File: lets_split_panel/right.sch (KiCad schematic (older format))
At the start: 52 parts, among them J5 Speaker, J6 ISP, J8 WS2812>, P5 USB_OTG, P6 >WS2812, P8 Conn_01x04, SW25 Socket, SW26 Socket, SW27 Socket, SW28 Socket, SW29 Socket, SW30 Socket, SW31 Socket, SW32 Socket, SW33 Socket, SW34 Socket, SW35 Socket, SW36 Socket, SW37 Socket, SW38 Socket, SW39 Socket, SW40 Socket, SW41 Socket, SW42 Socket, SW43 Socket, SW44 Socket, SW45 Socket, SW46 Socket, SW47 Socket, SW48 Socket, U2 ATMega32U4, Y2 Crystal

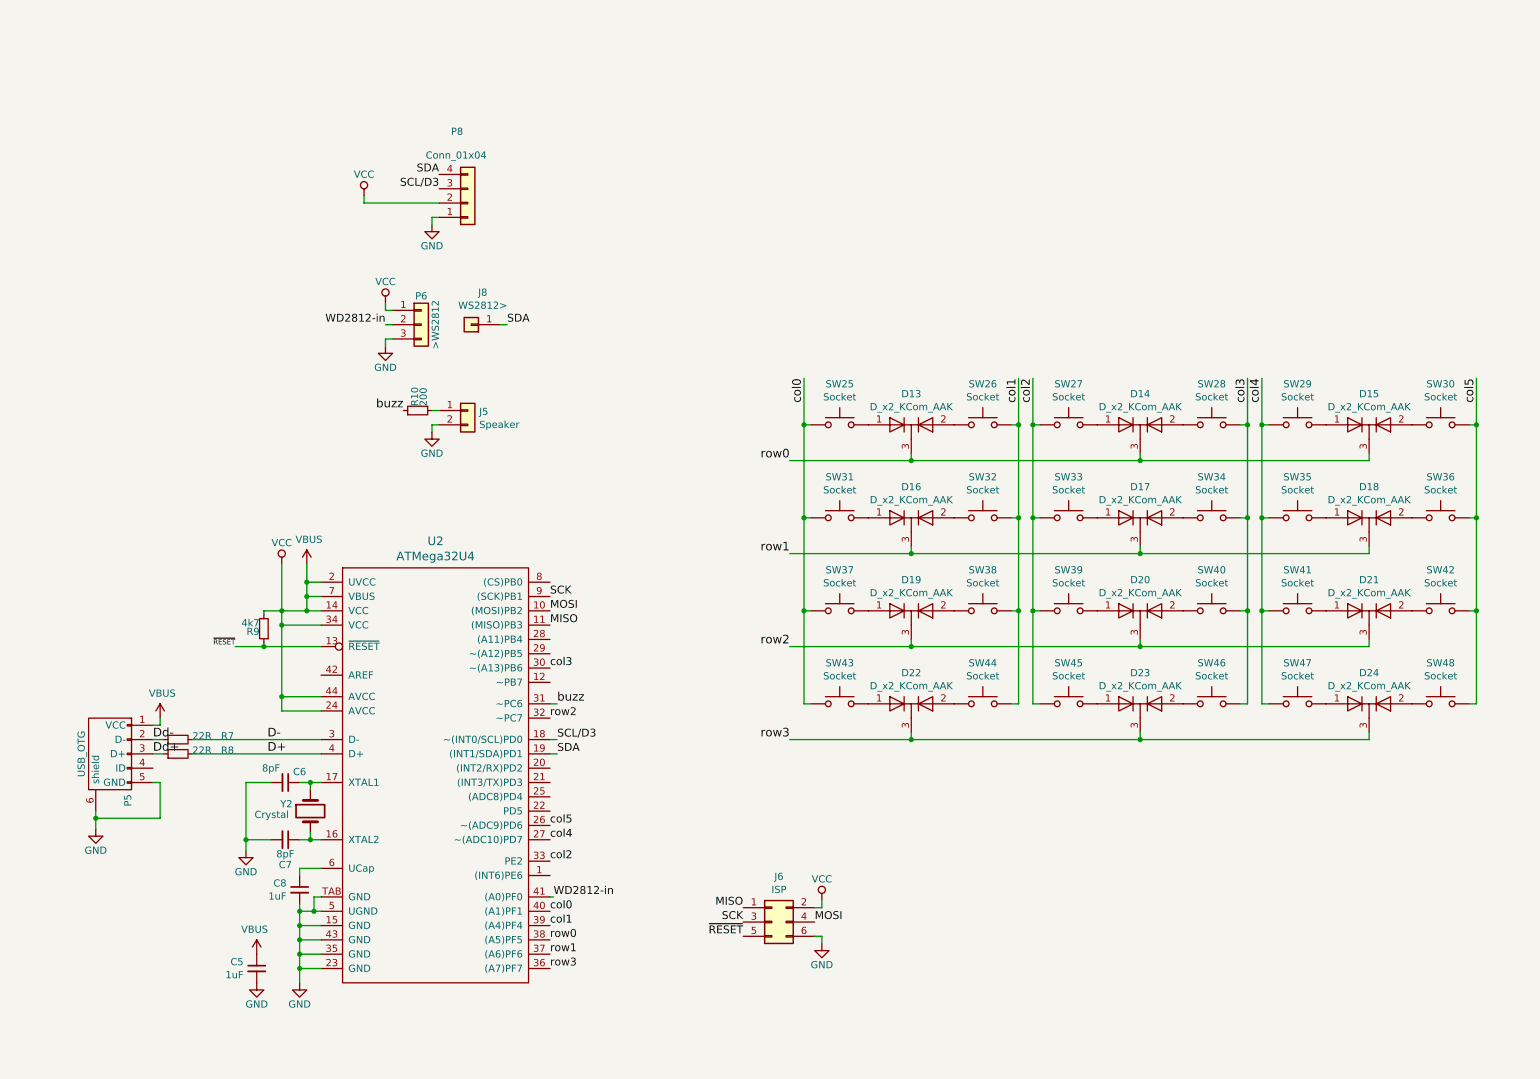
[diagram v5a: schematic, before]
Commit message: Added PnP files and split gerbers
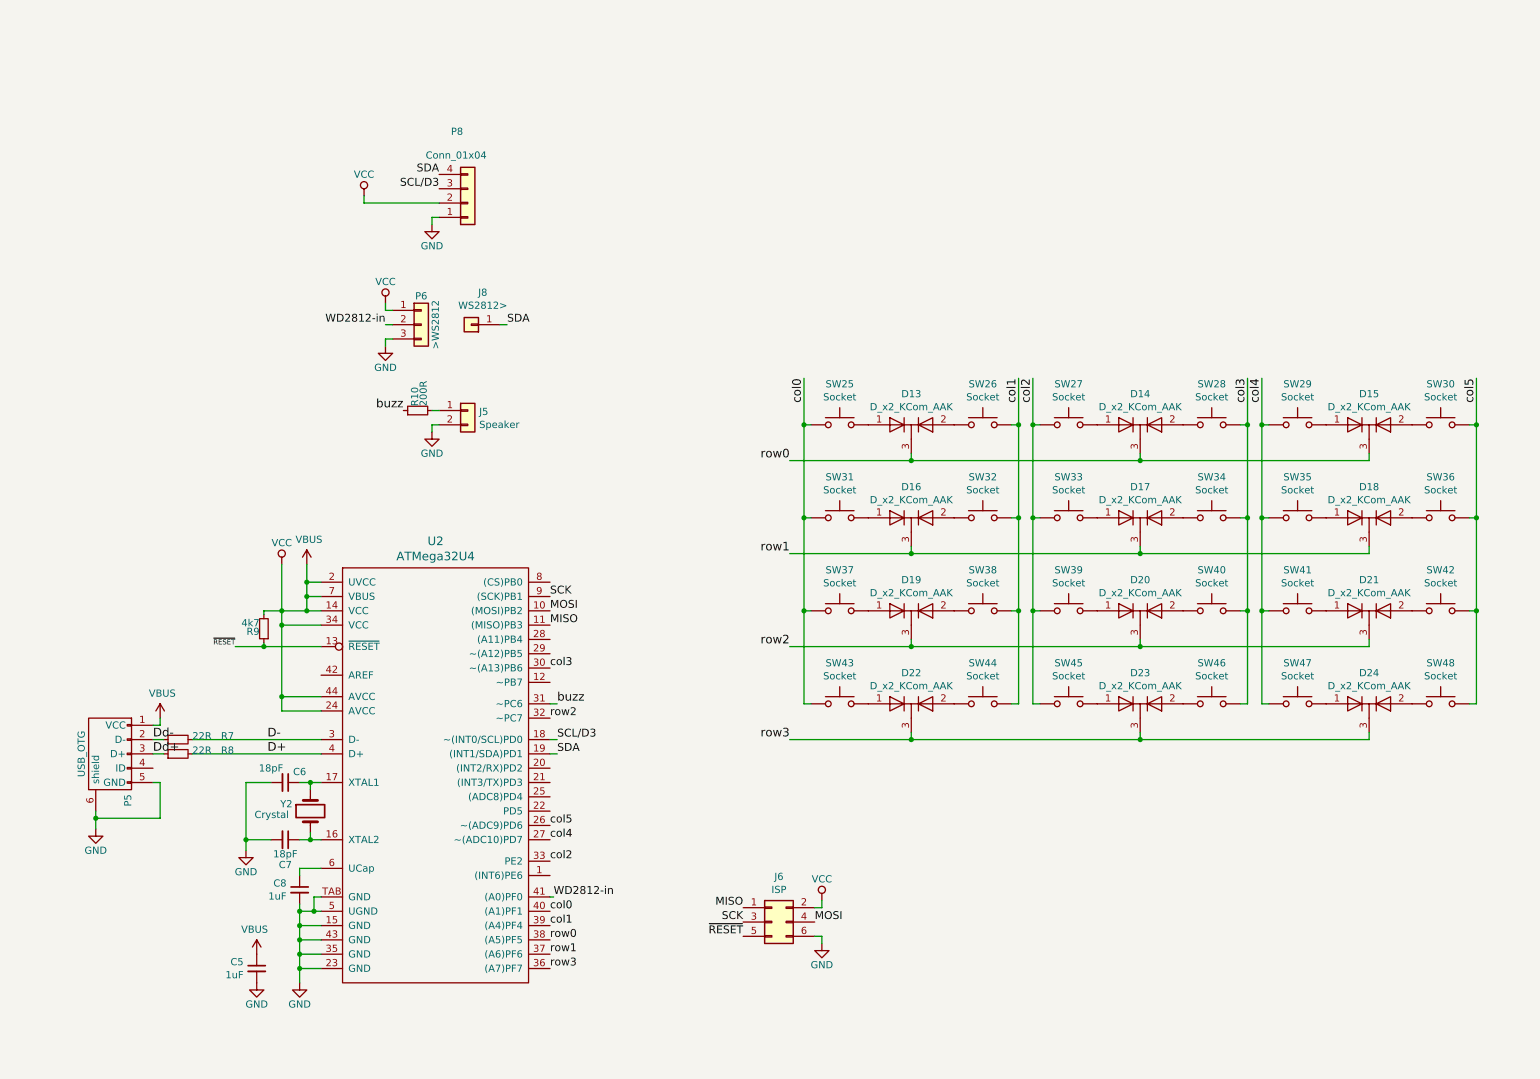
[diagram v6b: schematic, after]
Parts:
- C6, C7: value 8pF -> 18pF
- R10: value 200 -> 200R
- Y2: footprint SeeedOPL-Crystal Oscillator-2016:X2-SMD-3.2X1.5X0.55MM -> Crystals:Crystal_SMD_Abracon_ABM3-2pin_5.0x3.2mm
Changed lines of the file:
@@
 P 3300 3125
 F 0 "R10" H 3330 3145 50  0000 L CNN
-F 1 "200" H 3330 3085 50  0000 L CNN
+F 1 "200R" H 3330 3085 50  0000 L CNN
 F 2 "Resistors_SMD:R_0603" H 3300 3125 50  0001 C CNN
 F 3 "" H 3300 3125 50  0000 C CNN
@@
 F 0 "Y2" V 2500 6050 50  0000 L CNN
 F 1 "Crystal" V 2575 6075 50  0000 L CNN
-F 2 "SeeedOPL-Crystal Oscillator-2016:X2-SMD-3.2X1.5X0.55MM" H 2550 5925 50  0001 C CNN
+F 2 "Crystals:Crystal_SMD_Abracon_ABM3-2pin_5.0x3.2mm" H 2550 5925 50  0001 C CNN
 F 3 "" H 2550 5925 50  0001 C CNN
 	1    2550 5925
@@
 P 2375 5725
 F 0 "C6" V 2300 5825 50  0000 C CNN
-F 1 "8pF" V 2275 5625 50  0000 C CNN
+F 1 "18pF" V 2275 5625 50  0000 C CNN
 F 2 "Capacitors_SMD:C_0603" H 2375 5725 50  0001 C CNN
 F 3 "" H 2375 5725 50  0001 C CNN
@@
 P 2375 6125
 F 0 "C7" V 2550 6125 50  0000 C CNN
-F 1 "8pF" V 2475 6125 50  0000 C CNN
+F 1 "18pF" V 2475 6125 50  0000 C CNN
 F 2 "Capacitors_SMD:C_0603" H 2375 6125 50  0001 C CNN
 F 3 "" H 2375 6125 50  0001 C CNN
@@
 	2925 1675 3450 1675
 Wire Wire Line
-	2475 6575 2475 7125
+	2475 6575 2475 6625
 Wire Wire Line
 	2475 6925 2625 6925
@@
 Connection ~ 2475 6925
 Wire Wire Line
-	2225 4525 2625 4525
-Wire Wire Line
-	2350 4200 2350 5225
+	2225 4525 2350 4525
+Wire Wire Line
+	2350 4200 2350 4525
 Wire Wire Line
 	3400 1825 3400 1775
@@
 Connection ~ 2475 6825
 Wire Wire Line
-	2475 6625 2625 6625
+	2475 6625 2575 6625
 Connection ~ 2475 6725
 Wire Wire Line
@@
 	2550 5775 2550 5725
 Wire Wire Line
-	2475 5725 2625 5725
+	2475 5725 2550 5725
 Wire Wire Line
 	2550 6075 2550 6125
 Wire Wire Line
-	2475 6125 2625 6125
+	2475 6125 2550 6125
 Wire Wire Line
 	2225 4775 2225 4750
@@
 	2225 4525 2225 4550
 Wire Wire Line
-	2525 4200 2525 4525
+	2525 4200 2525 4325
 Wire Wire Line
 	2525 4425 2625 4425
@@
 	1500 5325 1500 5275
 Wire Wire Line
-	1050 5925 1050 6050
+	1050 5925 1050 5975
 Wire Wire Line
 	2100 5725 2275 5725
@@
 	2475 7025 2625 7025
 Wire Wire Line
-	2100 5725 2100 6200
+	2100 5725 2100 6125
 Wire Wire Line
 	1050 5975 1500 5975
@@
 	6050 3225 6000 3225
 Wire Wire Line
-	6000 2900 6000 5175
-Wire Wire Line
-	7500 2900 7500 5175
+	6000 2900 6000 3225
+Wire Wire Line
+	7500 2900 7500 3225
 Wire Wire Line
 	7500 3225 7450 3225
@@
 	6750 3425 6750 3475
 Wire Wire Line
-	5900 3475 9950 3475
+	5900 3475 6750 3475
 $Comp
 L device:D_x2_KCom_AAK D14
@@
 	7650 3225 7600 3225
 Wire Wire Line
-	7600 2900 7600 5175
-Wire Wire Line
-	9100 2900 9100 5175
+	7600 2900 7600 3225
+Wire Wire Line
+	9100 2900 9100 3225
 Wire Wire Line
 	9100 3225 9050 3225
@@
 	9250 3225 9200 3225
 Wire Wire Line
-	9200 2900 9200 5175
-Wire Wire Line
-	10700 2900 10700 5175
+	9200 2900 9200 3225
+Wire Wire Line
+	10700 2900 10700 3225
 Wire Wire Line
 	10700 3225 10650 3225
@@
 	6750 4075 6750 4125
 Wire Wire Line
-	5900 4125 9950 4125
+	5900 4125 6750 4125
 $Comp
 L device:D_x2_KCom_AAK D17
@@
 	6750 4725 6750 4775
 Wire Wire Line
-	5900 4775 9950 4775
+	5900 4775 6750 4775
 $Comp
 L device:D_x2_KCom_AAK D20
@@
 	6750 5375 6750 5425
 Wire Wire Line
-	5900 5425 9950 5425
+	5900 5425 6750 5425
 $Comp
 L device:D_x2_KCom_AAK D23
@@
 Connection ~ 10700 3225
 Wire Wire Line
-	2025 4775 2625 4775
+	2025 4775 2225 4775
+Wire Wire Line
+	2475 7025 2475 7125
+Wire Wire Line
+	2475 6925 2475 7025
+Wire Wire Line
+	2475 6825 2475 6925
+Wire Wire Line
+	2475 6725 2475 6825
+Wire Wire Line
+	2350 4525 2525 4525
+Wire Wire Line
+	2350 4525 2350 4625
+Wire Wire Line
+	2350 4625 2350 5125
+Wire Wire Line
+	2350 5125 2350 5225
+Wire Wire Line
+	2225 4775 2625 4775
+Wire Wire Line
+	2525 4325 2525 4425
+Wire Wire Line
+	2475 6625 2475 6725
+Wire Wire Line
+	2550 6125 2625 6125
+Wire Wire Line
+	2550 5725 2625 5725
+Wire Wire Line
+	2100 6125 2100 6200
+Wire Wire Line
+	1050 5975 1050 6050
+Wire Wire Line
+	2575 6625 2625 6625
+Wire Wire Line
+	2525 4525 2625 4525
+Wire Wire Line
+	2525 4425 2525 4525
+Wire Wire Line
+	6750 3475 8350 3475
+Wire Wire Line
+	8350 3475 9950 3475
+Wire Wire Line
+	6750 4125 8350 4125
+Wire Wire Line
+	8350 4125 9950 4125
+Wire Wire Line
+	6750 4775 8350 4775
+Wire Wire Line
+	8350 4775 9950 4775
+Wire Wire Line
+	6750 5425 8350 5425
+Wire Wire Line
+	8350 5425 9950 5425
+Wire Wire Line
+	6000 4525 6000 5175
+Wire Wire Line
+	6000 3875 6000 4525
+Wire Wire Line
+	6000 3225 6000 3875
+Wire Wire Line
+	7500 3225 7500 3875
+Wire Wire Line
+	7600 3225 7600 3875
+Wire Wire Line
+	7500 3875 7500 4525
+Wire Wire Line
+	7600 3875 7600 4525
+Wire Wire Line
+	7500 4525 7500 5175
+Wire Wire Line
+	7600 4525 7600 5175
+Wire Wire Line
+	9100 3225 9100 3875
+Wire Wire Line
+	9100 3875 9100 4525
+Wire Wire Line
+	9100 4525 9100 5175
+Wire Wire Line
+	9200 4525 9200 5175
+Wire Wire Line
+	9200 3875 9200 4525
+Wire Wire Line
+	9200 3225 9200 3875
+Wire Wire Line
+	10700 4525 10700 5175
+Wire Wire Line
+	10700 3875 10700 4525
+Wire Wire Line
+	10700 3225 10700 3875
 $EndSCHEMATC

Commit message: Added BOM
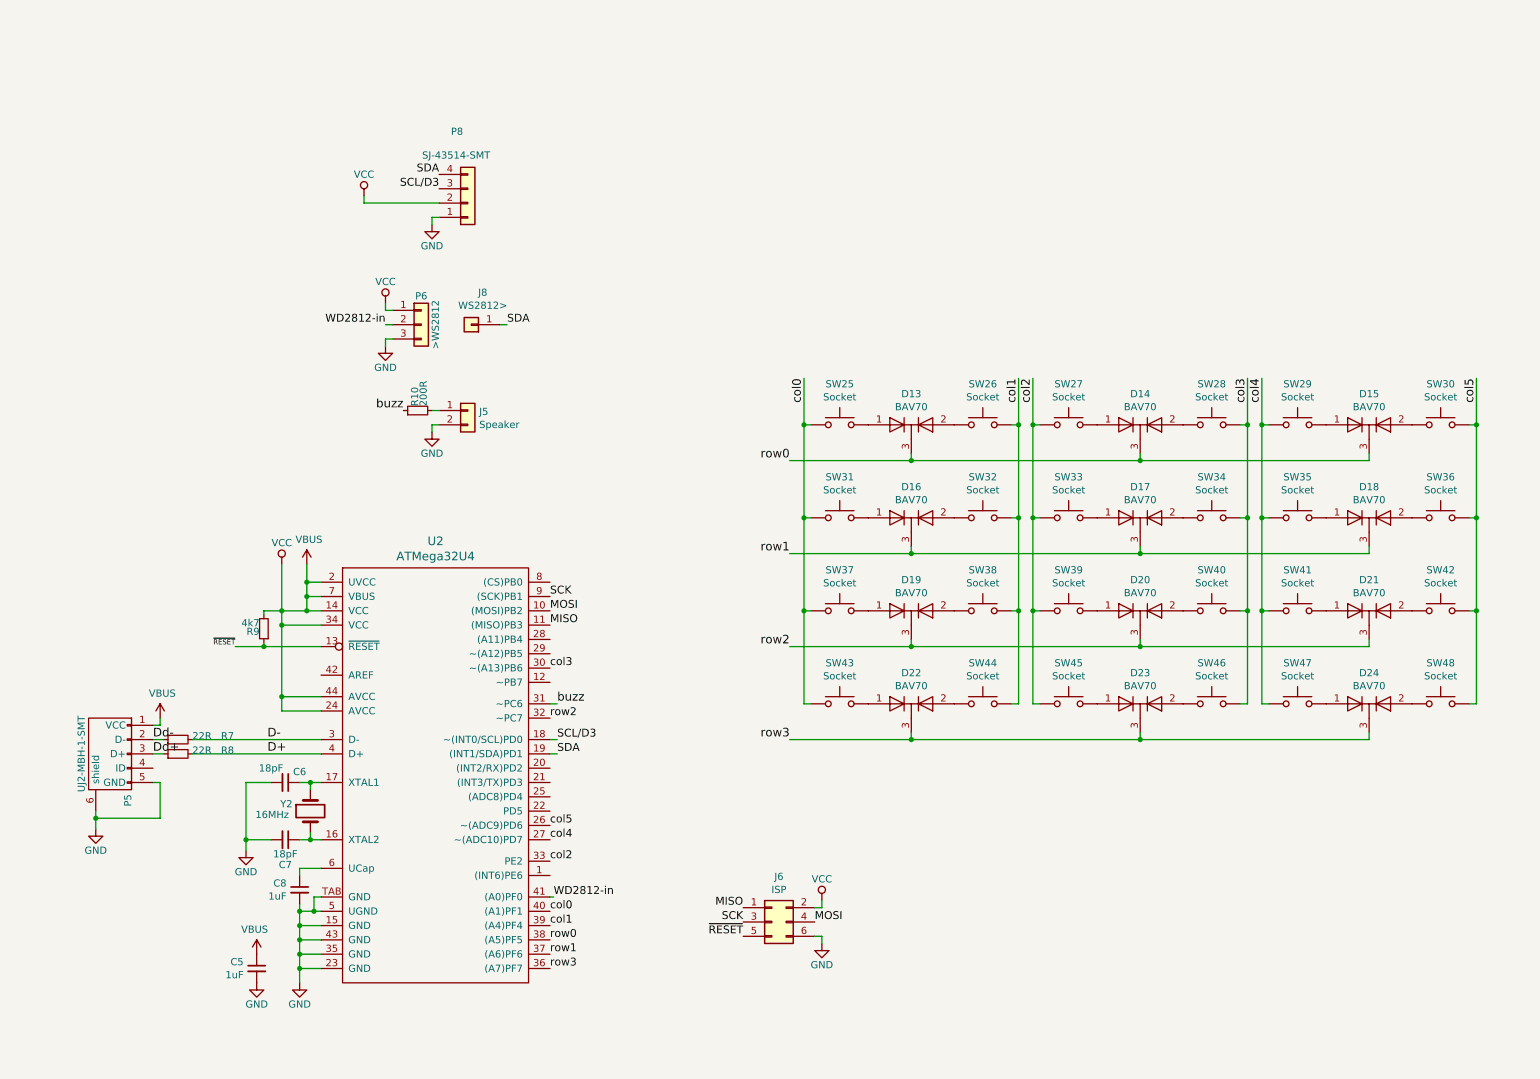
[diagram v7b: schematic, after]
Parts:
- D13, D14, D15, D16, D17, D18, D19, D20, D21, D22, D23, D24: value D_x2_KCom_AAK -> BAV70
- P5: value USB_OTG -> UJ2-MBH-1-SMT
- P8: value Conn_01x04 -> SJ-43514-SMT
- Y2: value Crystal -> 16MHz
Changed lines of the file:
@@
 P 1150 5525
 F 0 "P5" H 1475 5400 50  0000 C CNN
-F 1 "USB_OTG" H 1150 5725 50  0000 C CNN
+F 1 "UJ2-MBH-1-SMT" H 1150 5725 50  0000 C CNN
 F 2 "Connectors:USB-Mini-B-SMD" V 1100 5425 50  0001 C CNN
 F 3 "" V 1100 5425 50  0000 C CNN
@@
 P 3650 1675
 F 0 "P8" H 3575 1175 50  0000 C CNN
-F 1 "Conn_01x04" H 3569 1341 50  0000 C CNN
+F 1 "SJ-43514-SMT" H 3569 1341 50  0000 C CNN
 F 2 "Connectors:SJ-4351X-SMT" H 3650 1675 50  0001 C CNN
 F 3 "" H 3650 1675 50  0001 C CNN
@@
 P 2550 5925
 F 0 "Y2" V 2500 6050 50  0000 L CNN
-F 1 "Crystal" V 2575 6075 50  0000 L CNN
+F 1 "16MHz" V 2575 6075 50  0000 L CNN
 F 2 "Crystals:Crystal_SMD_Abracon_ABM3-2pin_5.0x3.2mm" H 2550 5925 50  0001 C CNN
 F 3 "" H 2550 5925 50  0001 C CNN
@@
 P 6750 3225
 F 0 "D13" H 6750 3441 50  0000 C CNN
-F 1 "D_x2_KCom_AAK" H 6750 3350 50  0000 C CNN
+F 1 "BAV70" H 6750 3350 50  0000 C CNN
 F 2 "TO_SOT_Packages_SMD:SOT-23" H 6750 3225 50  0001 C CNN
 F 3 "" H 6750 3225 50  0001 C CNN
@@
 P 8350 3225
 F 0 "D14" H 8350 3441 50  0000 C CNN
-F 1 "D_x2_KCom_AAK" H 8350 3350 50  0000 C CNN
+F 1 "BAV70" H 8350 3350 50  0000 C CNN
 F 2 "TO_SOT_Packages_SMD:SOT-23" H 8350 3225 50  0001 C CNN
 F 3 "" H 8350 3225 50  0001 C CNN
@@
 P 9950 3225
 F 0 "D15" H 9950 3441 50  0000 C CNN
-F 1 "D_x2_KCom_AAK" H 9950 3350 50  0000 C CNN
+F 1 "BAV70" H 9950 3350 50  0000 C CNN
 F 2 "TO_SOT_Packages_SMD:SOT-23" H 9950 3225 50  0001 C CNN
 F 3 "" H 9950 3225 50  0001 C CNN
@@
 P 6750 3875
 F 0 "D16" H 6750 4091 50  0000 C CNN
-F 1 "D_x2_KCom_AAK" H 6750 4000 50  0000 C CNN
+F 1 "BAV70" H 6750 4000 50  0000 C CNN
 F 2 "TO_SOT_Packages_SMD:SOT-23" H 6750 3875 50  0001 C CNN
 F 3 "" H 6750 3875 50  0001 C CNN
@@
 P 8350 3875
 F 0 "D17" H 8350 4091 50  0000 C CNN
-F 1 "D_x2_KCom_AAK" H 8350 4000 50  0000 C CNN
+F 1 "BAV70" H 8350 4000 50  0000 C CNN
 F 2 "TO_SOT_Packages_SMD:SOT-23" H 8350 3875 50  0001 C CNN
 F 3 "" H 8350 3875 50  0001 C CNN
@@
 P 9950 3875
 F 0 "D18" H 9950 4091 50  0000 C CNN
-F 1 "D_x2_KCom_AAK" H 9950 4000 50  0000 C CNN
+F 1 "BAV70" H 9950 4000 50  0000 C CNN
 F 2 "TO_SOT_Packages_SMD:SOT-23" H 9950 3875 50  0001 C CNN
 F 3 "" H 9950 3875 50  0001 C CNN
@@
 P 6750 4525
 F 0 "D19" H 6750 4741 50  0000 C CNN
-F 1 "D_x2_KCom_AAK" H 6750 4650 50  0000 C CNN
+F 1 "BAV70" H 6750 4650 50  0000 C CNN
 F 2 "TO_SOT_Packages_SMD:SOT-23" H 6750 4525 50  0001 C CNN
 F 3 "" H 6750 4525 50  0001 C CNN
@@
 P 8350 4525
 F 0 "D20" H 8350 4741 50  0000 C CNN
-F 1 "D_x2_KCom_AAK" H 8350 4650 50  0000 C CNN
+F 1 "BAV70" H 8350 4650 50  0000 C CNN
 F 2 "TO_SOT_Packages_SMD:SOT-23" H 8350 4525 50  0001 C CNN
 F 3 "" H 8350 4525 50  0001 C CNN
@@
 P 9950 4525
 F 0 "D21" H 9950 4741 50  0000 C CNN
-F 1 "D_x2_KCom_AAK" H 9950 4650 50  0000 C CNN
+F 1 "BAV70" H 9950 4650 50  0000 C CNN
 F 2 "TO_SOT_Packages_SMD:SOT-23" H 9950 4525 50  0001 C CNN
 F 3 "" H 9950 4525 50  0001 C CNN
@@
 P 6750 5175
 F 0 "D22" H 6750 5391 50  0000 C CNN
-F 1 "D_x2_KCom_AAK" H 6750 5300 50  0000 C CNN
+F 1 "BAV70" H 6750 5300 50  0000 C CNN
 F 2 "TO_SOT_Packages_SMD:SOT-23" H 6750 5175 50  0001 C CNN
 F 3 "" H 6750 5175 50  0001 C CNN
@@
 P 8350 5175
 F 0 "D23" H 8350 5391 50  0000 C CNN
-F 1 "D_x2_KCom_AAK" H 8350 5300 50  0000 C CNN
+F 1 "BAV70" H 8350 5300 50  0000 C CNN
 F 2 "TO_SOT_Packages_SMD:SOT-23" H 8350 5175 50  0001 C CNN
 F 3 "" H 8350 5175 50  0001 C CNN
@@
 P 9950 5175
 F 0 "D24" H 9950 5391 50  0000 C CNN
-F 1 "D_x2_KCom_AAK" H 9950 5300 50  0000 C CNN
+F 1 "BAV70" H 9950 5300 50  0000 C CNN
 F 2 "TO_SOT_Packages_SMD:SOT-23" H 9950 5175 50  0001 C CNN
 F 3 "" H 9950 5175 50  0001 C CNN
